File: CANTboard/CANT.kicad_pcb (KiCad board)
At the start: 2 copper layers, 35.1 x 50 mm, 41 parts, among them J1 Screw_Terminal_01x04, P1 SWD, P3 USB, U1 STM32H743VITx, U2 MCP2558FD-xSN, U3 LD1117S33TR, U4 74LVC1G66, U5 74LVC1G66, U6 MCP2558FD-xSN

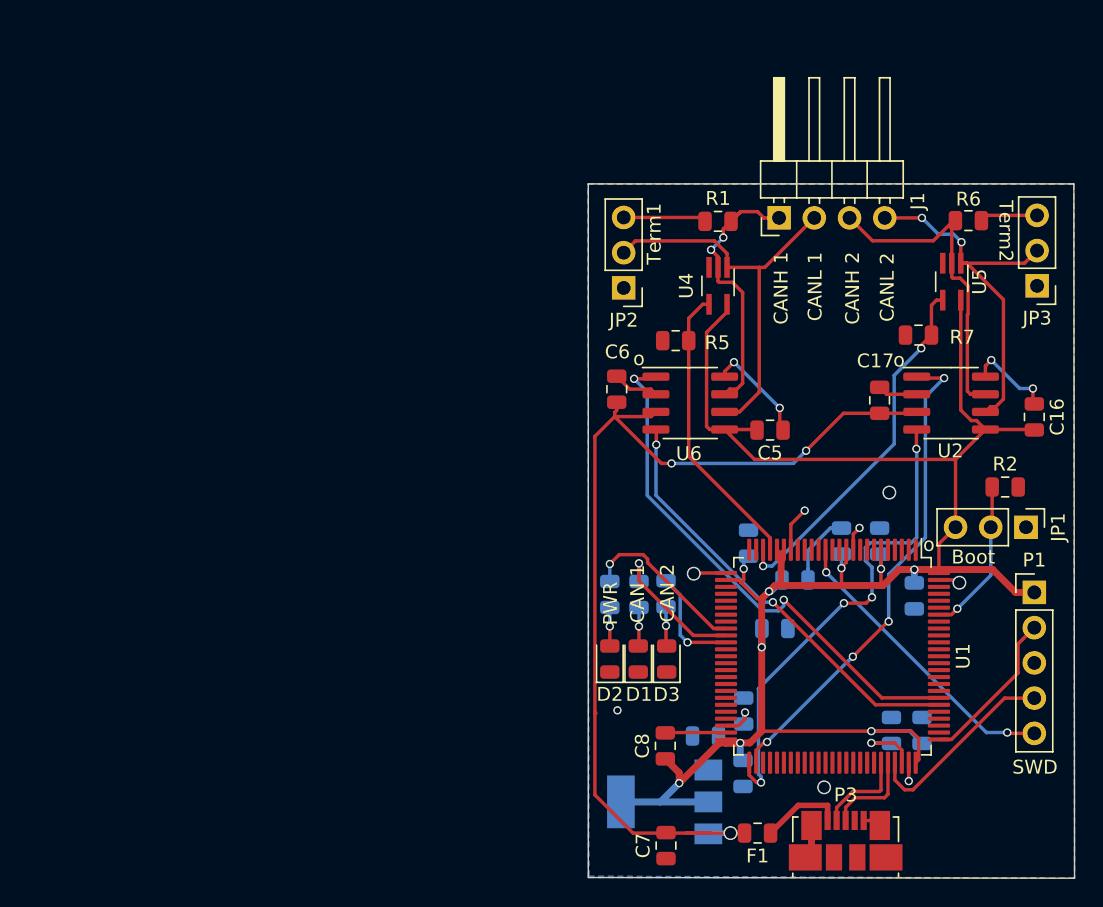
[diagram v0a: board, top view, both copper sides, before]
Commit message: Starting design of unified board
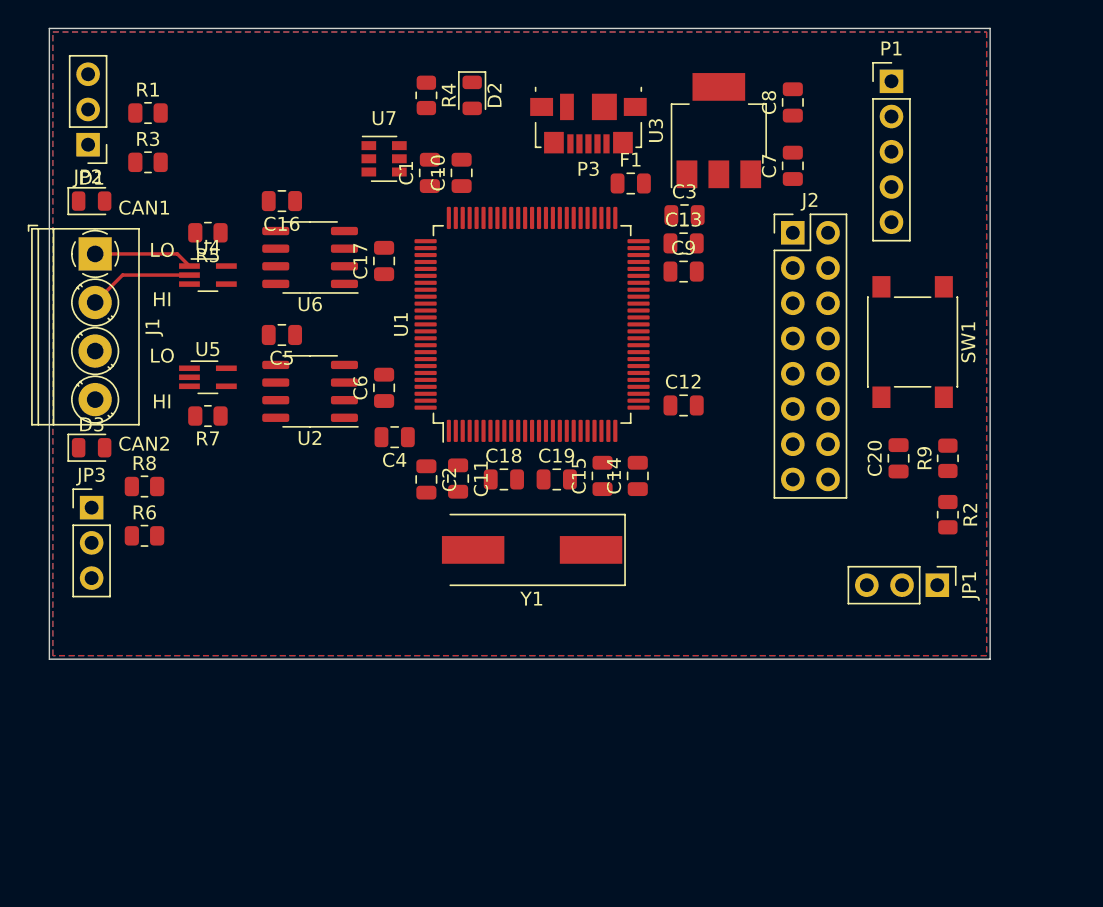
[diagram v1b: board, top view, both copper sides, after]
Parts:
- added C18: 26pF, Capacitor_SMD:C_0805_2012Metric, F.Cu at (105.7, 98.8)
- added C19: 26pF, Capacitor_SMD:C_0805_2012Metric, F.Cu at (109.5, 98.8)
- added C20: 100nF, Capacitor_SMD:C_0805_2012Metric, F.Cu at (134.1, 97.3)
- added J2: Conn_02x08_Odd_Even, Connector_PinHeader_2.54mm:PinHeader_2x08_P2.54mm_Vertical, F.Cu at (126.5, 81.0)
- added R9: 100K, Resistor_SMD:R_0805_2012Metric, F.Cu at (137.7, 97.3)
- added SW1: SW_SPST, Button_Switch_SMD:SW_SPST_PTS645, F.Cu at (135.1, 88.9)
- added U7: USBLC6-2SC6, Package_TO_SOT_SMD:SOT-23-6, F.Cu at (97.0, 75.7)
- added Y1: Crystal, Crystal:Crystal_SMD_HC49-SD, F.Cu at (107.7, 103.9)
- C1, C10, C11, C12, C13, C14, C15, C2, C3, C4, C9, R3, R4, R8: moved to F.Cu
- J1: footprint Connector_PinHeader_2.54mm:PinHeader_1x04_P2.54mm_Horizontal -> TerminalBlock_Phoenix:TerminalBlock_Phoenix_PT-1,5-4-3.5-H_1x04_P3.50mm_Horizontal
- U3: footprint TO_SOT_Packages_SMD:SOT-223 -> Package_TO_SOT_SMD:SOT-223; moved to F.Cu
- moved JP3 70.0 mm to (75.9, 100.8), turned to 0 degrees
- moved R6 63.6 mm to (79.8, 102.9), turned to 0 degrees
- moved C16 56.4 mm to (89.7, 78.7), turned to 180 degrees
- moved P3 54.9 mm to (111.8, 73.2), turned to 180 degrees
- moved U5 54.1 mm to (84.3, 91.4), turned to 0 degrees
- moved R7 51.6 mm to (84.3, 94.2)
- moved D1 51.4 mm to (75.9, 78.7), turned to 0 degrees
- moved C10 50.7 mm to (102.6, 76.7)
- moved C7 49.8 mm to (126.5, 76.2), turned to 90 degrees
- moved J1 49.4 mm to (76.2, 82.5), turned to 270 degrees
- moved U3 48.5 mm to (121.2, 73.7), turned to 90 degrees
- moved F1 47.7 mm to (114.8, 77.5), turned to 0 degrees
- moved C8 47.3 mm to (126.5, 71.6)
- moved R3 47.1 mm to (80.0, 75.9), turned to 0 degrees
- moved U2 46.2 mm to (91.7, 92.5), turned to 180 degrees
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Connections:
- J1 pad 1: CAN1_H -> CAN1_L
- J1 pad 2: CAN1_L -> CAN1_H
- J1 pad 3: CAN2_H -> CAN2_L
- J1 pad 4: CAN2_L -> CAN2_H
- JP1 pad 1: (no net) -> Net-(JP1-Pad1)
- JP2 pad 1: (no net) -> Net-(JP2-Pad1)
- JP3 pad 1: (no net) -> Net-(JP3-Pad1)
- P3 pad 4: (no net) -> Net-(P3-Pad4)
- U1 pad 1: (no net) -> Net-(U1-Pad1)
- U1 pad 12: (no net) -> Net-(C18-Pad2)
- U1 pad 13: (no net) -> Net-(C19-Pad1)
- U1 pad 15: (no net) -> Net-(U1-Pad15)
- U1 pad 16: (no net) -> Net-(U1-Pad16)
- U1 pad 17: (no net) -> Net-(U1-Pad17)
- U1 pad 18: (no net) -> Net-(U1-Pad18)
- U1 pad 2: (no net) -> Net-(U1-Pad2)
- U1 pad 22: CAN1_SHORT -> Net-(U1-Pad22)
- U1 pad 23: CAN2_SHORT -> Net-(U1-Pad23)
- U1 pad 24: (no net) -> Net-(U1-Pad24)
- U1 pad 25: (no net) -> Net-(U1-Pad25)
- U1 pad 28: (no net) -> Net-(U1-Pad28)
- U1 pad 29: (no net) -> Net-(U1-Pad29)
- U1 pad 3: (no net) -> Net-(U1-Pad3)
- U1 pad 30: (no net) -> Net-(U1-Pad30)
- U1 pad 31: (no net) -> Net-(U1-Pad31)
- U1 pad 32: (no net) -> Net-(U1-Pad32)
- U1 pad 33: (no net) -> Net-(U1-Pad33)
- U1 pad 37: (no net) -> Net-(U1-Pad37)
- U1 pad 38: (no net) -> Net-(J2-Pad15)
- U1 pad 39: (no net) -> Net-(J2-Pad13)
- U1 pad 4: (no net) -> Net-(U1-Pad4)
- U1 pad 40: (no net) -> Net-(J2-Pad11)
- U1 pad 41: (no net) -> Net-(J2-Pad9)
- U1 pad 42: (no net) -> Net-(J2-Pad7)
- U1 pad 43: (no net) -> Net-(J2-Pad5)
- U1 pad 44: (no net) -> Net-(J2-Pad3)
- U1 pad 45: (no net) -> Net-(J2-Pad1)
- U1 pad 46: (no net) -> Net-(U1-Pad46)
- U1 pad 47: (no net) -> Net-(U1-Pad47)
- U1 pad 5: (no net) -> Net-(U1-Pad5)
- U1 pad 51: /CAN2_RX -> Net-(U1-Pad51)
- U1 pad 52: /CAN2_TX -> Net-(U1-Pad52)
- U1 pad 53: (no net) -> Net-(U1-Pad53)
- U1 pad 54: (no net) -> Net-(U1-Pad54)
- U1 pad 55: (no net) -> Net-(U1-Pad55)
- U1 pad 56: (no net) -> Net-(U1-Pad56)
- U1 pad 57: (no net) -> Net-(U1-Pad57)
- U1 pad 58: (no net) -> Net-(U1-Pad58)
- U1 pad 59: (no net) -> Net-(U1-Pad59)
- U1 pad 60: (no net) -> Net-(U1-Pad60)
- U1 pad 61: (no net) -> Net-(U1-Pad61)
- U1 pad 62: (no net) -> Net-(U1-Pad62)
- U1 pad 63: (no net) -> Net-(U1-Pad63)
- U1 pad 64: (no net) -> Net-(U1-Pad64)
- U1 pad 65: (no net) -> Net-(U1-Pad65)
- U1 pad 66: (no net) -> Net-(U1-Pad66)
- U1 pad 67: (no net) -> Net-(U1-Pad67)
- U1 pad 68: (no net) -> Net-(U1-Pad68)
- U1 pad 69: (no net) -> Net-(U1-Pad69)
- U1 pad 7: (no net) -> Net-(U1-Pad7)
- U1 pad 77: (no net) -> Net-(U1-Pad77)
- U1 pad 78: (no net) -> Net-(U1-Pad78)
- U1 pad 79: (no net) -> Net-(U1-Pad79)
- U1 pad 8: (no net) -> Net-(U1-Pad8)
- U1 pad 80: (no net) -> Net-(U1-Pad80)
- U1 pad 81: /CAN1_RX -> Net-(U1-Pad81)
- U1 pad 82: /CAN1_TX -> Net-(U1-Pad82)
- U1 pad 83: (no net) -> Net-(U1-Pad83)
- U1 pad 84: (no net) -> Net-(U1-Pad84)
- U1 pad 85: (no net) -> Net-(U1-Pad85)
- U1 pad 86: (no net) -> Net-(U1-Pad86)
- U1 pad 87: (no net) -> Net-(U1-Pad87)
- U1 pad 88: (no net) -> Net-(U1-Pad88)
- U1 pad 89: (no net) -> Net-(U1-Pad89)
- U1 pad 9: (no net) -> Net-(U1-Pad9)
- U1 pad 90: (no net) -> CAN2_SHORT
- U1 pad 91: (no net) -> CAN2_RX
- U1 pad 92: (no net) -> CAN2_TX
- U1 pad 93: (no net) -> CAN1_SHORT
- U1 pad 95: (no net) -> CAN1_RX
- U1 pad 96: (no net) -> CAN1_TX
- U1 pad 97: (no net) -> Net-(U1-Pad97)
- U1 pad 98: (no net) -> Net-(U1-Pad98)
- U2 pad 1: /CAN2_TX -> CAN2_TX
- U2 pad 4: /CAN2_RX -> CAN2_RX
- U6 pad 1: /CAN1_TX -> CAN1_TX
- U6 pad 4: /CAN1_RX -> CAN1_RX
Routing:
- net VCC: track 147.9 -> 0.00 mm, vias 9 -> 0
- net VBUS: track 72.2 -> 0.00 mm, vias 3 -> 0
- net GND: track 43.9 -> 0.00 mm, vias 12 -> 0
- net /CAN1_TX: track 38.4 -> 0.00 mm, vias 2 -> 0
- net /CAN2_TX: track 35.5 -> 0.00 mm, vias 4 -> 0
- net /CAN2_RX: track 35.4 -> 0.00 mm, vias 4 -> 0
- net /CAN1_RX: track 31.4 -> 0.00 mm, vias 2 -> 0
- net CAN2_L: track 26.7 -> 0.00 mm, vias 2 -> 0
- net CAN2_SHORT: track 26.4 -> 0.00 mm, vias 2 -> 0
- net CAN2_H: track 24.5 -> 0.00 mm
- net CAN1_L: track 29.0 -> 7.16 mm
- net /NRST: track 21.5 -> 0.00 mm, vias 2 -> 0
- net CAN1_SHORT: track 21.0 -> 0.00 mm
- net /SWDIO: track 14.3 -> 0.00 mm
- net CAN1_H: track 20.3 -> 7.62 mm, vias 2 -> 0
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- added copper zone on B.Cu, net VCC
- removed copper zone on B.Cu, net GND
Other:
- board size 35.1 x 50 mm -> 67.8 x 45.5 mm
- board text added: "CAN1"
- board text added: "CAN2"
- board text added: "HI"
- board text added: "LO"
- board text removed: "1. 3.3v 2. SWCLK 3. GND 4. SWDIO 5. NRST"
- board text removed: "Boot"
- board text removed: "CAN 1"
- board text removed: "CAN 2"
- board text removed: "CANH 1"
- board text removed: "CANH 2"
- board text removed: "CANL 1"
- board text removed: "CANL 2"
- board text removed: "PWR"
- board text removed: "SWD"
- board text removed: "Term1"
- board text removed: "Term2"
- board text removed: "Version: 1.0"
- board text removed: "https://github.com/bitbane/CANT Tim Brom Managing Senior Security Researcher @b1tbane thb@grimm-co.com"
- board text removed: "o"

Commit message: Finished layout, ordered first set of prototype boards
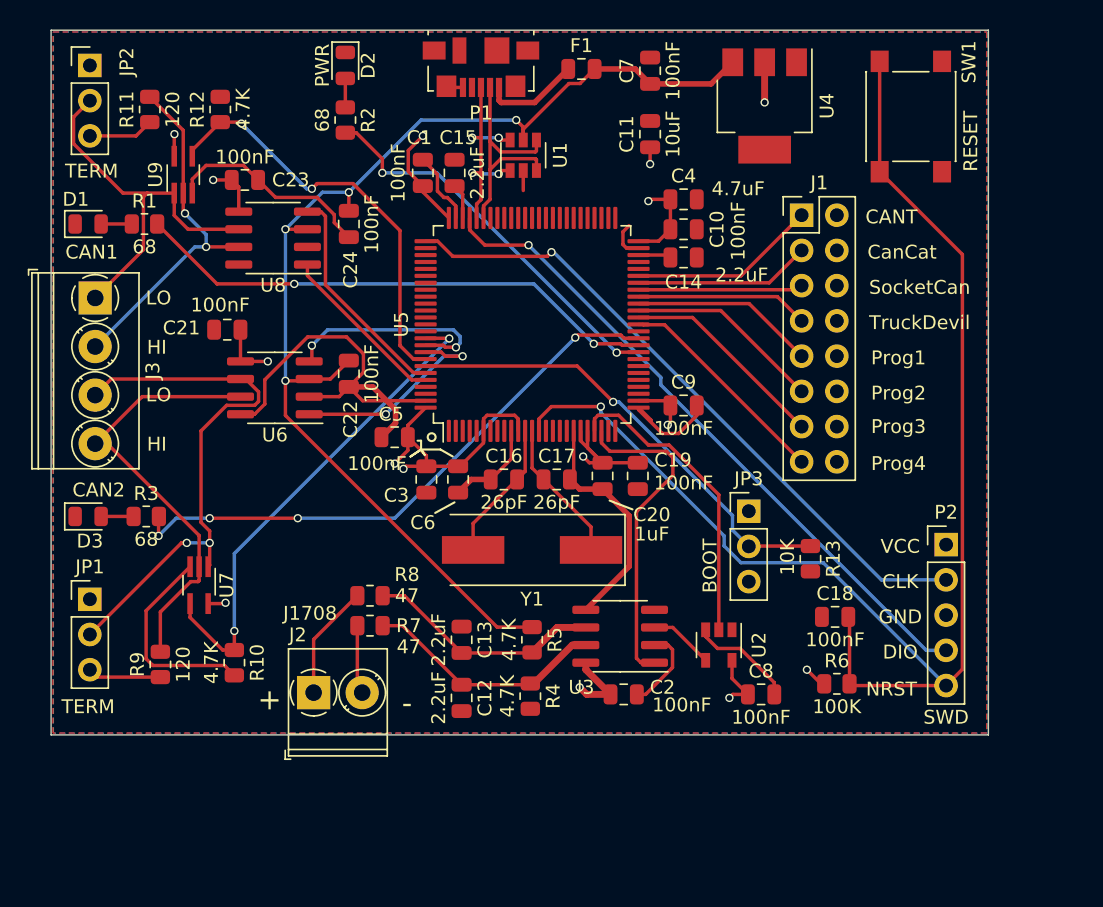
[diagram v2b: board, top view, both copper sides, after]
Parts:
- removed the C3 at (118.7, 79.8)
- removed the C6 at (97.0, 92.2)
- removed the C9 at (118.6, 83.8)
- removed the R1 at (80.0, 72.4)
- removed the R2 at (137.7, 101.3)
- removed the U4 at (84.3, 84.1)
- removed the U7 at (97.0, 75.7)
- added C10: 100nF, Capacitor_SMD:C_0805_2012Metric, F.Cu at (118.6, 80.8)
- added C11: 10uF, Capacitor_SMD:C_0805_2012Metric, F.Cu at (116.2, 73.9)
- added C12: 2.2uF, Capacitor_SMD:C_0805_2012Metric, F.Cu at (102.6, 114.6)
- added C14: 2.2uF, Capacitor_SMD:C_0805_2012Metric, F.Cu at (118.6, 82.8)
- added C2: 100nF, Capacitor_SMD:C_0805_2012Metric, F.Cu at (114.3, 114.3)
- added C22: 100nF, Capacitor_SMD:C_0805_2012Metric, F.Cu at (94.5, 91.2)
- added C4: 4.7uF, Capacitor_SMD:C_0805_2012Metric, F.Cu at (118.6, 78.6)
- added G***: LOGO, KiCad:Logo, B.Cu at (115.3, 89.7)
- added J2: Screw_Terminal_01x02, TerminalBlock_Phoenix:TerminalBlock_Phoenix_PT-1,5-2-3.5-H_1x02_P3.50mm_Horizontal, F.Cu at (91.9, 114.2)
- added R11: 120, Resistor_SMD:R_0805_2012Metric, F.Cu at (80.1, 72.1)
- added R13: 10k, Resistor_SMD:R_0805_2012Metric, F.Cu at (127.8, 104.5)
- added R4: 4.7K, Resistor_SMD:R_0805_2012Metric, F.Cu at (107.6, 114.4)
- added R5: 4.7K, Resistor_SMD:R_0805_2012Metric, F.Cu at (107.7, 110.4)
- added R7: 47, Resistor_SMD:R_0805_2012Metric, F.Cu at (96.0, 109.3)
- added R8: 47, Resistor_SMD:R_0805_2012Metric, F.Cu at (96.0, 107.2)
- added U1: USBLC6-2SC6, Package_TO_SOT_SMD:SOT-23-6, F.Cu at (107.1, 75.4)
- added U2: SN74LVC1G14DBV, Package_TO_SOT_SMD:SOT-23-5, F.Cu at (121.2, 110.7)
- added U3: ST485EBDR, Package_SO:SOIC-8_3.9x4.9mm_P1.27mm, F.Cu at (114.0, 110.1)
- added U9: 74LVC1G66, Package_TO_SOT_SMD:SOT-353_SC-70-5_Handsoldering, F.Cu at (82.5, 76.8)
- C13: value 100nF -> 2.2uF
- C8: value 10uF -> 100nF
- moved C8 42.7 mm to (124.2, 114.3), turned to 0 degrees
- moved P2 33.6 mm to (137.5, 103.5)
- moved C13 32.8 mm to (102.6, 110.4), turned to 270 degrees
- moved R6 18.1 mm to (129.7, 113.5), turned to 0 degrees
- moved R10 17.9 mm to (86.2, 112.0), turned to 270 degrees
- moved SW1 16.3 mm to (135.0, 72.6)
- moved U7 15.0 mm to (83.7, 106.4), turned to 270 degrees
- moved JP3 14.6 mm to (123.3, 101.1), turned to 0 degrees
- moved C7 12.4 mm to (116.2, 69.3)
- moved C18 12.3 mm to (129.5, 108.7), turned to 0 degrees
- moved D2 9.40 mm to (94.2, 69.0)
- moved R9 9.34 mm to (80.9, 112.1), turned to 90 degrees
- moved F1 8.99 mm to (111.3, 69.2)
- moved R12 8.93 mm to (85.2, 72.1), turned to 90 degrees
- moved P1 8.75 mm to (104.0, 69.1)
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- renumbered C10 to C15, C18 to C16, C19 to C17, C20 to C18, C14 to C19, C15 to C20, C5 to C21, C16 to C23, C17 to C24, C2 to C3, C4 to C5, C11 to C6, C12 to C9, J2 to J1, J1 to J3, JP3 to JP1, JP1 to JP3, P3 to P1, P1 to P2, R3 to R1, R7 to R10, R5 to R12, R4 to R2, R8 to R3, R9 to R6, R6 to R9, U3 to U4, U1 to U5, U2 to U6, U5 to U7, U6 to U8
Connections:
- C13 pad 1: VCC -> GND
- C13 pad 2: GND -> Net-(C13-Pad2)
- U5 pad 22: Net-(U1-Pad22) -> J1708_TX
- U5 pad 23: Net-(U1-Pad23) -> J1708_RX
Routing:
- net GND: track 0.00 -> 117.1 mm
- net /NRST: track 0.00 -> 99.4 mm, vias 0 -> 1
- net VBUS: track 0.00 -> 85.9 mm, vias 0 -> 4
- net VCC: track 0.00 -> 73.8 mm, vias 0 -> 15
- net /SWDIO: track 0.00 -> 48.1 mm, vias 0 -> 1
- net /SWCLK: track 0.00 -> 47.9 mm, vias 0 -> 1
- net LED_ACT2: track 0.00 -> 42.1 mm, vias 0 -> 4
- net CAN2_L: track 0.00 -> 39.8 mm, vias 0 -> 2
- net LED_ACT1: track 0.00 -> 38.3 mm, vias 0 -> 2
- net CAN2_SHORT: track 0.00 -> 35.7 mm, vias 0 -> 2
- net BOOT0: track 0.00 -> 33.8 mm, vias 0 -> 1
- net CAN2_H: track 0.00 -> 32.0 mm
- net CAN1_SHORT: track 0.00 -> 30.3 mm, vias 0 -> 2
- net LED_PWR1: track 0.00 -> 28.3 mm, vias 0 -> 2
- net J1708_RX: track 0.00 -> 23.4 mm
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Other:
- board size 67.8 x 45.5 mm -> 67.6 x 50.8 mm
- board text added: "+"
- board text added: "-"
- board text added: "100K"
- board text added: "100nF"
- board text added: "10K"
- board text added: "10uF"
- board text added: "120"
- board text added: "1uF"
- board text added: "2.2uF"
- board text added: "26pF"
- board text added: "4.7K"
- board text added: "4.7uF"
- board text added: "47"
- board text added: "68"
- board text added: "BOOT"
- board text added: "CANT"
- board text added: "CLK"
- board text added: "CanCat"
- board text added: "DIO"
- board text added: "GND"
- board text added: "J1708"
- board text added: "NRST"
- board text added: "One Board To Run Them All https://github.com/bitbane/CANT @b1tbane"
- board text added: "PWR"
- board text added: "Prog1"
- board text added: "Prog2"
- board text added: "Prog3"
- board text added: "Prog4"
- board text added: "RESET"
- board text added: "SWD"
- board text added: "SocketCan"
- board text added: "TERM"
- board text added: "TruckDevil"
- board text added: "VCC"
